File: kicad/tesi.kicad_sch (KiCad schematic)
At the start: 34 parts, among them J1 Conn_01x04_Pin, J2 Conn_01x04_Pin, J3 Conn_01x04_Pin, J4 Conn_01x04_Pin, SW1 POWER, U1 MAX4466, U2 BNO055, U3 MPR121, U4 VL53L1CX

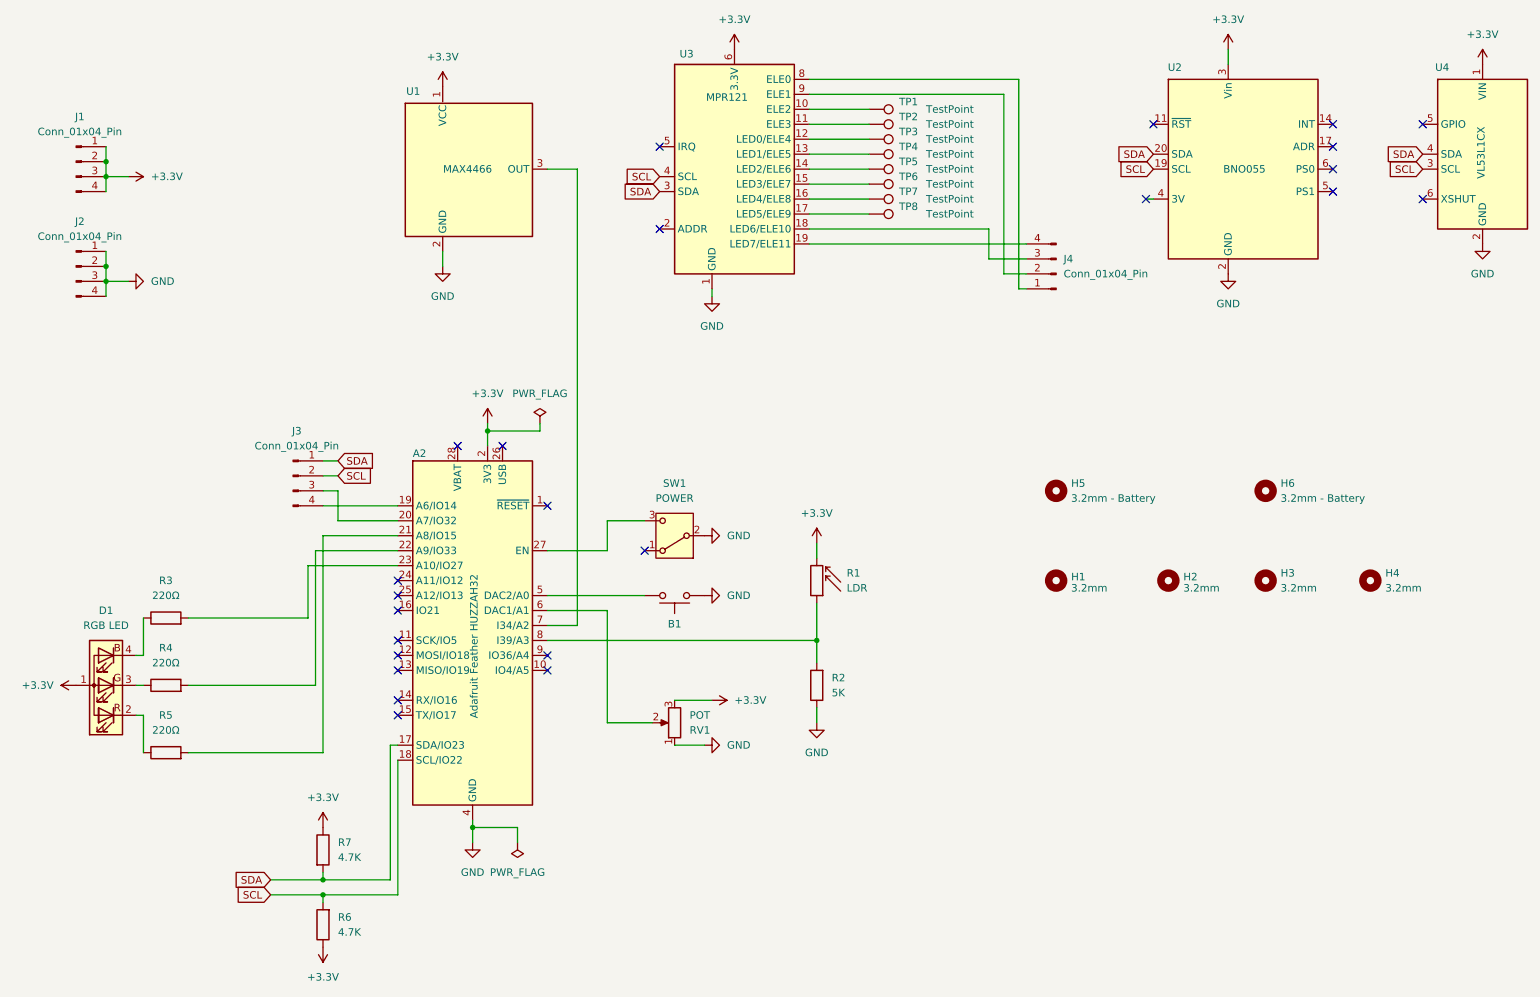
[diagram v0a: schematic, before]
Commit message: update pcb
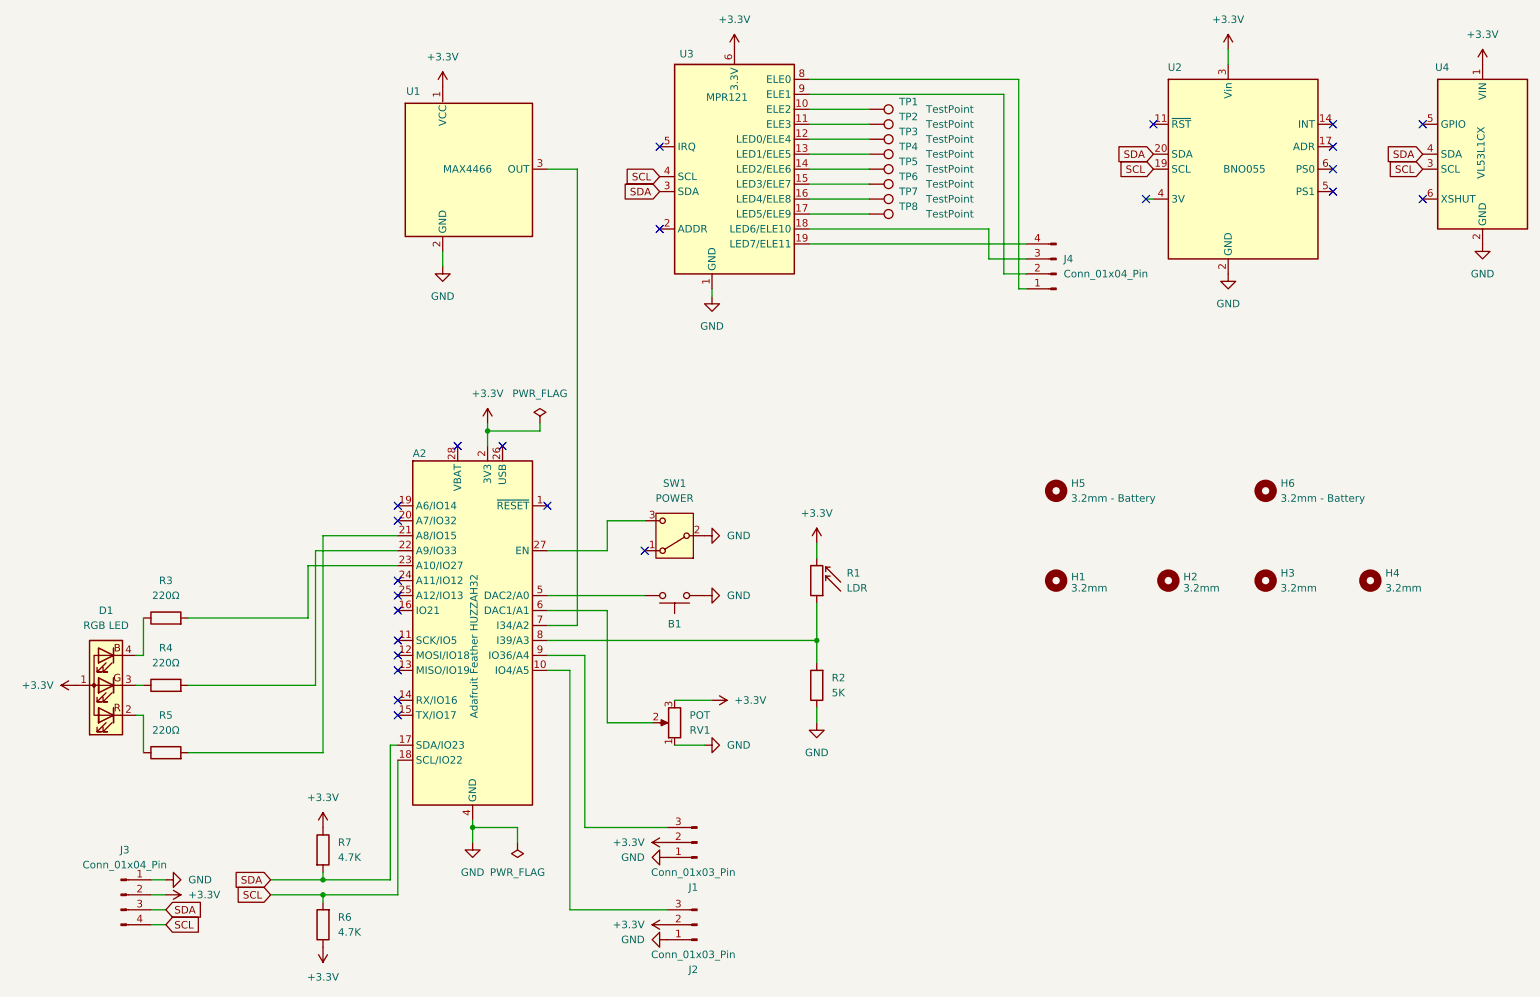
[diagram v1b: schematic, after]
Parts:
- removed J1, J2: Conn_01x04_Pin, Connector_PinSocket_2.54mm:PinSocket_1x04_P2.54mm_Vertical, symbol Connector:Conn_01x04_Pin
- added J1, J2: Conn_01x03_Pin, Connector_PinSocket_2.54mm:PinSocket_1x03_P2.54mm_Vertical, symbol Connector:Conn_01x03_Pin
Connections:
- net +3.3V: now also J3.2 (Pin_2), J1.2 (Pin_2), J2.2 (Pin_2)
- net GND: now also J3.1 (Pin_1), J1.1 (Pin_1), J2.1 (Pin_1)
- net SCL: now also J3.4 (Pin_4); no longer J3.2 (Pin_2)
- net SDA: now also J3.3 (Pin_3); no longer J3.1 (Pin_1)
- net at A2.20 (A7/IO32): no longer J3.3 (Pin_3)
- net at A2.19 (A6/IO14): no longer J3.4 (Pin_4)
- net at A2.10 (IO4/A5): now also J2.3 (Pin_3)
- net at A2.9 (IO36/A4): now also J1.3 (Pin_3)
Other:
- moved on the sheet: J3
